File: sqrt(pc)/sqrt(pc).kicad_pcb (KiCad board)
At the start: 4 copper layers, 64 x 41.5 mm, 32 parts, among them J1 Conn_01x02, Q1 AO3401A, U1 WEMOSC3mini, U2 TP4056-42-ESOP8

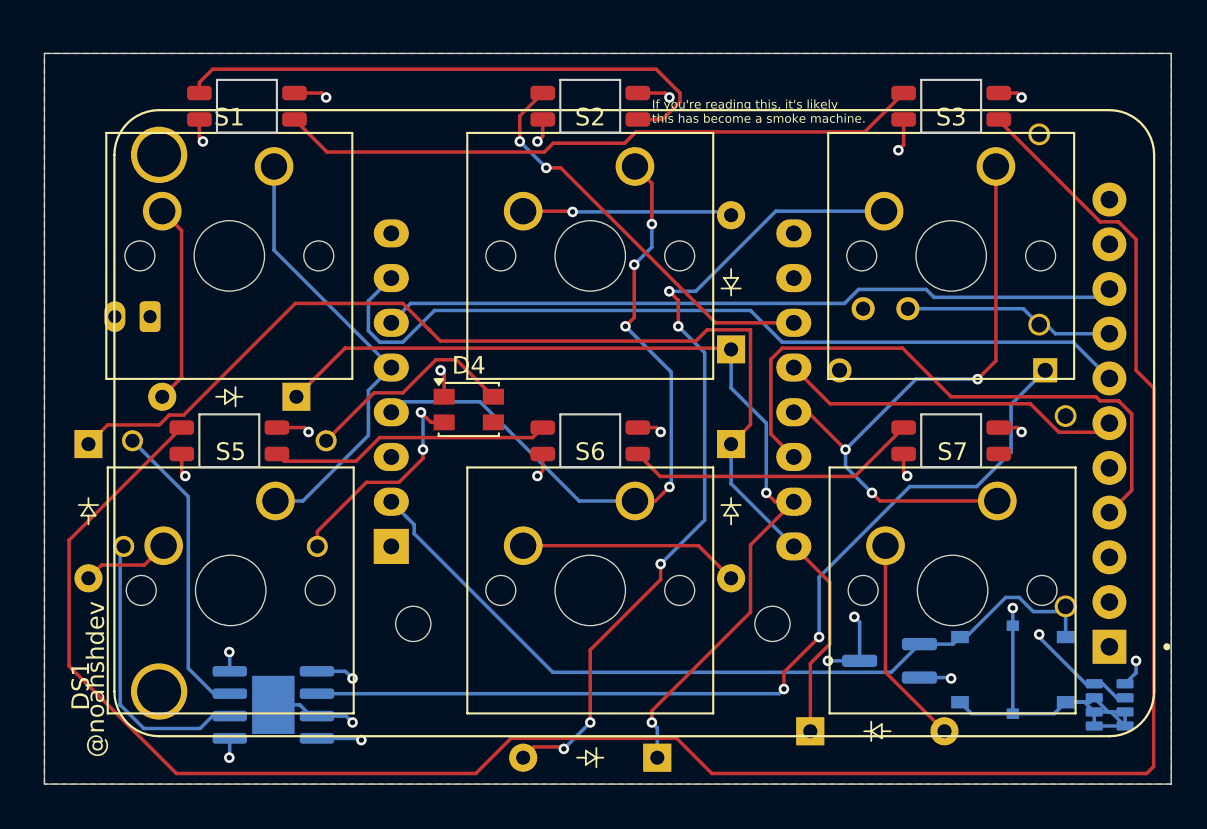
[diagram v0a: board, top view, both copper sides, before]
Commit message: BOM + a lot more I guess
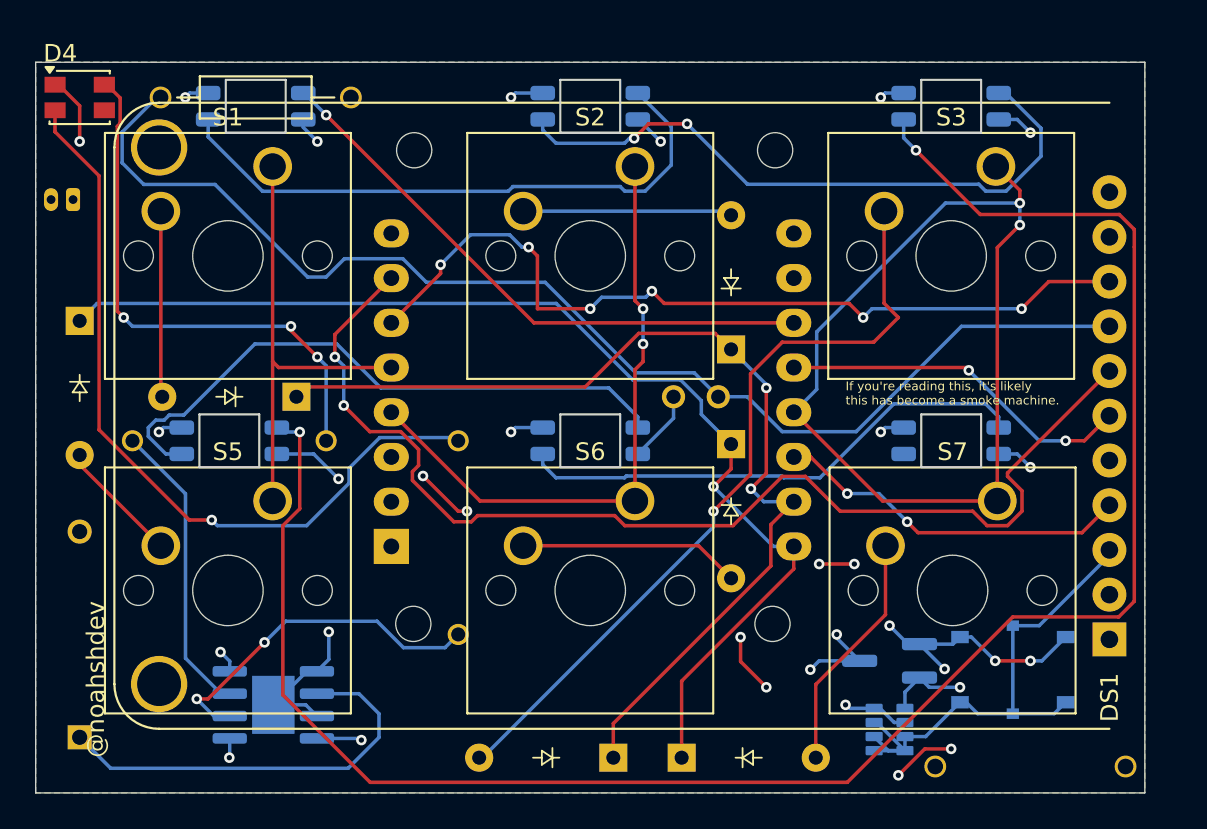
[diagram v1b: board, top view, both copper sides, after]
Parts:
- D10, D11, D12, D13, D14, D9: moved to B.Cu
- J1: footprint Connector_JST:JST_PH_B2B-PH-K_1x02_P2.00mm_Vertical -> Connector_Molex:Molex_PicoBlade_53048-0210_1x02_P1.25mm_Horizontal
- R5: moved to F.Cu
- moved R2 58.7 mm to (33.5, 55.8), turned to 90 degrees
- moved R5 45.1 mm to (43.5, 19.5), turned to 180 degrees
- moved D4 28.3 mm to (33.5, 19.5)
- moved R6 14.6 mm to (87.5, 57.5), turned to 180 degrees
- moved R3 13.5 mm to (55.0, 44.5), turned to -90 degrees
- moved RN1 12.6 mm to (79.5, 55.4)
- moved C46 11.9 mm to (68.5, 36.5)
- moved J1 7.96 mm to (33.1, 25.3)
- moved D7 7.46 mm to (67.7, 57.0)
- moved D5 7.02 mm to (33.5, 32.2)
- moved D3 2.50 mm to (63.8, 57.0)
- moved D9 0.50 mm to (43.5, 20.0), turned to 180 degrees
- moved DS1 0.42 mm to (65.0, 37.6)
- moved S5 0.16 mm to (44.5, 42.4)
- moved S1 0.08 mm to (44.5, 23.4)
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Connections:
- D10 pad 4: LED_DIN -> Net-(D10-DIN)
- D11 pad 4: Net-(D11-DIN) -> Net-(D10-DOUT)
- D9 pad 2: Net-(D11-DIN) -> Net-(D10-DIN)
- D9 pad 4: Net-(D10-DOUT) -> LED_DIN
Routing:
- net BAT+: track 171.5 -> 106.9 mm, vias 3 -> 4
- net Net-(DS1-~{RST}): track 12.0 -> 70.5 mm
- net Net-(D11-DIN): track 36.8 -> 0.00 mm
- net Net-(D10-DIN): track 0.00 -> 34.3 mm
- net Net-(D4-GK): track 12.8 -> 44.5 mm, vias 2 -> 1
- net Net-(U2-PROG): track 53.1 -> 23.8 mm, vias 2 -> 0
- net 3V3: track 186.3 -> 215.5 mm
- net 5V-VBus: track 86.9 -> 58.6 mm
- net Net-(D12-DOUT): track 16.1 -> 34.9 mm
- net Net-(D4-RK): track 12.3 -> 30.9 mm, vias 0 -> 3
- net GND: track 197.8 -> 216.1 mm, vias 9 -> 6
- net Col 2: track 35.9 -> 53.4 mm, vias 3 -> 2
- net CS: track 48.2 -> 65.3 mm, vias 0 -> 2
- net BAT_ADC: track 51.3 -> 36.2 mm, vias 1 -> 5
- net Net-(D11-DOUT): track 123.2 -> 108.8 mm, vias 0 -> 2
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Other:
- board size 64 x 41.5 mm -> 63 x 41.5 mm
